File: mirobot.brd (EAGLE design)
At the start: 55.6 x 39 mm, 11 parts, among them X1 5_PIN_STEPPER, X2 5_PIN_STEPPER

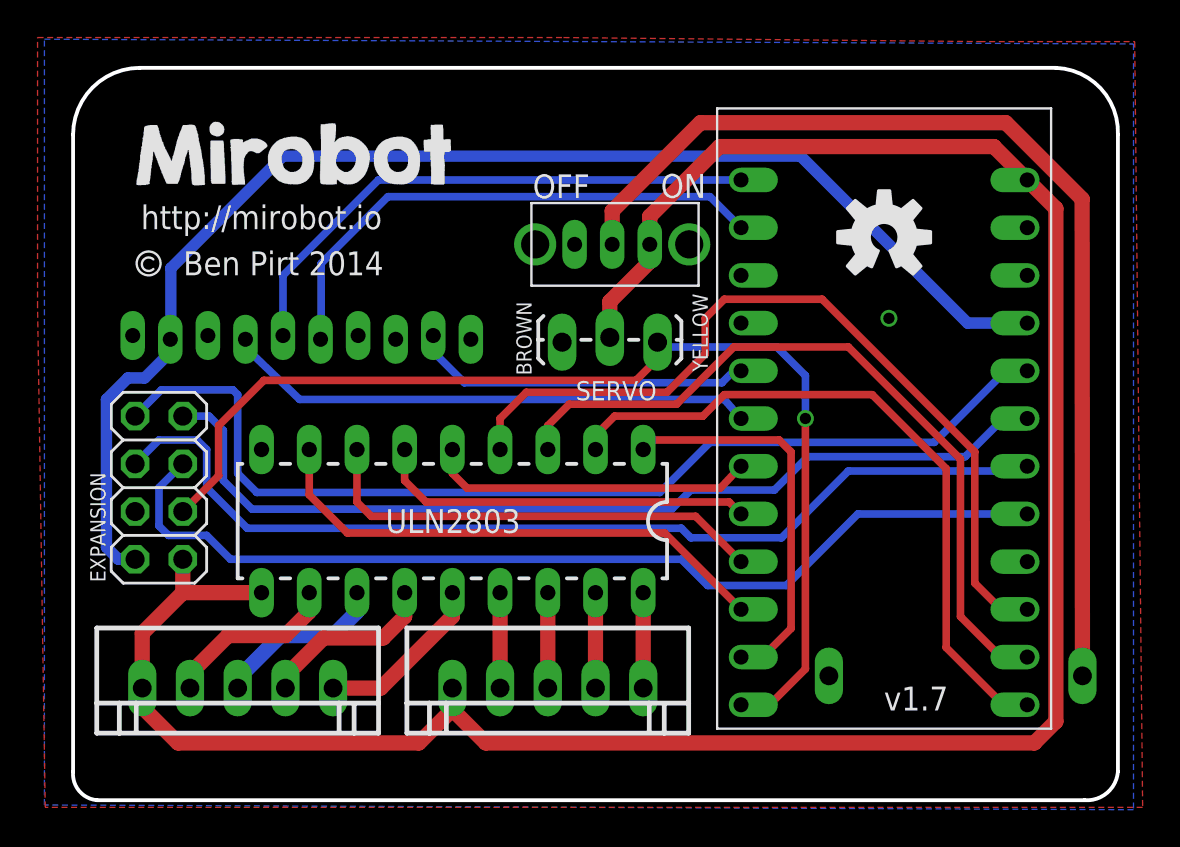
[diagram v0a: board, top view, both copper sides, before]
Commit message: v1.8 boards
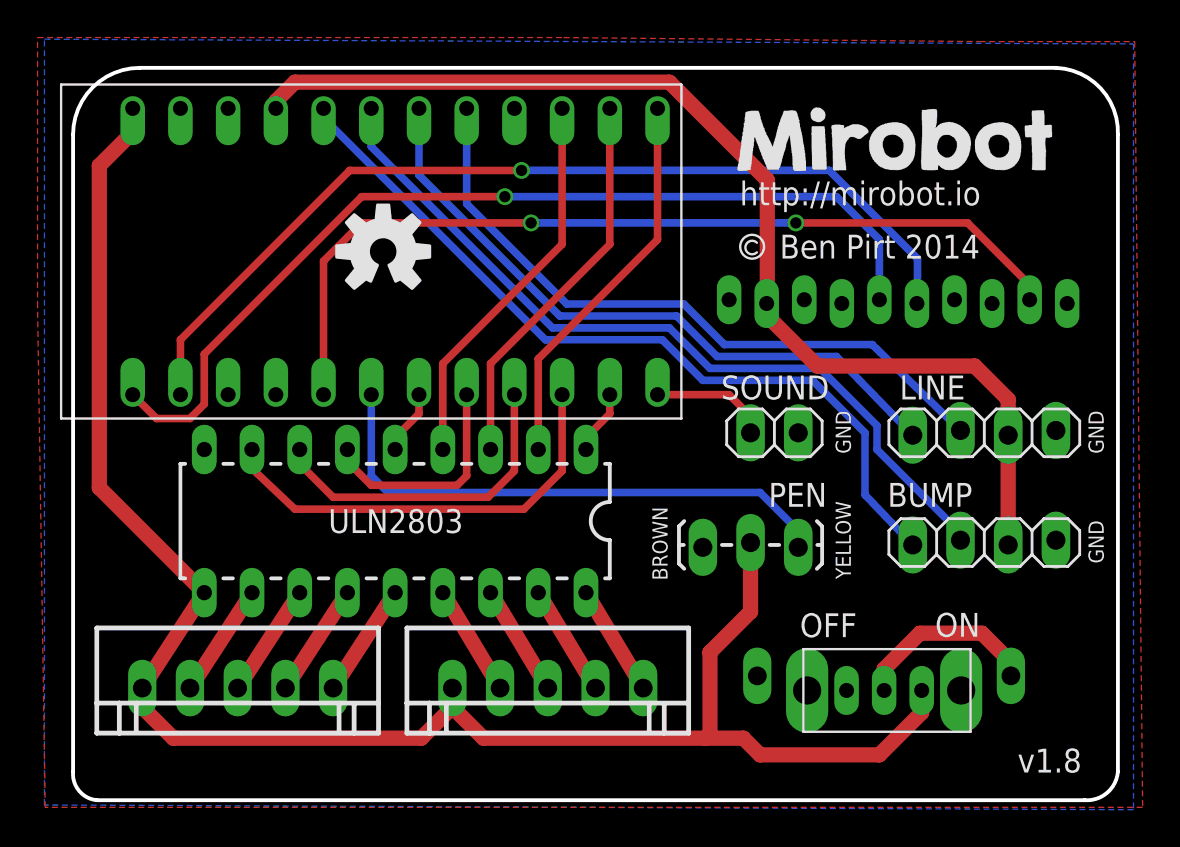
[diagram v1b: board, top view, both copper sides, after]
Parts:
- removed EXPANSION: (no value), pinhead:2X04
- removed SERVO: (no value), SparkFun-Connectors:1X03_LOCK_LONGPADS
- added BUMP, LINE: (no value), Child-Friendly-Parts:1X04
- added PEN: (no value), SparkFun-Connectors:1X03_LOCK_LONGPADS
- added SOUND: (no value), pinhead:1X02
- moved U$5 32.0 mm to (52.5, 50.7)
- moved U$1 31.8 mm to (51.8, 42.3)
- moved U$2 28.7 mm to (24.8, 45.0), turned to 90 degrees
- moved U$3 27.8 mm to (52.1, 21.6)
- moved LOGO1 26.7 mm to (25.4, 45.0)
- moved U$4 3.81 mm to (59.8, 23.4)
- moved ULN2803 3.05 mm to (26.0, 30.6)
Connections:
- removed net WIFI_RESET: U$1.EXT_RESET, U$2.D3
- new net SPEAKER: SOUND.2, U$2.D9
- net +3V3: now also BUMP.3, LINE.3; no longer EXPANSION.2
- net GND: now also BUMP.4, LINE.4, PEN.3, SOUND.1; no longer EXPANSION.4, SERVO.3
- net PC0: now also LINE.2; no longer EXPANSION.5
- net PC1: now also LINE.1; no longer EXPANSION.6
- net PC2: now also BUMP.2; no longer EXPANSION.7
- net PC3: now also BUMP.1; no longer EXPANSION.8
- net SERVO: now also PEN.1, U$2.D3; no longer EXPANSION.3, SERVO.1, U$2.D9
- net VSS: now also PEN.2; no longer EXPANSION.1, SERVO.2
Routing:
- net N$6: track 55.8 -> 10.0 mm
- net SERVO: track 59.5 -> 29.1 mm, vias 1 -> 0
- net VSS: track 124.6 -> 94.4 mm
- net NREADY: track 18.4 -> 47.7 mm, vias 0 -> 2
- net WIFI_RESET: track 28.4 -> 0.00 mm
- net MOTOR1_4: track 44.4 -> 20.8 mm
- net RXD: track 28.6 -> 50.2 mm, vias 0 -> 1
- net TXD: track 29.7 -> 50.9 mm, vias 0 -> 1
- net MOTOR1_3: track 40.3 -> 20.8 mm
- net MOTOR1_1: track 21.3 -> 3.45 mm
- net PC1: track 52.9 -> 35.6 mm
- net PC0: track 52.9 -> 36.3 mm
- net MOTOR1_2: track 37.1 -> 20.8 mm
- net MOTOR2_1: track 17.5 -> 3.45 mm
- net PC3: track 55.5 -> 43.3 mm
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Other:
- board text added: "GND"
- board text added: "v1.8"
- board text removed: "v1.7"
